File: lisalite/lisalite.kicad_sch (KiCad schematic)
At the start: 4 parts, among them U1 74LS85, U2 74LS393, U3 74LS85, U4 74LS74

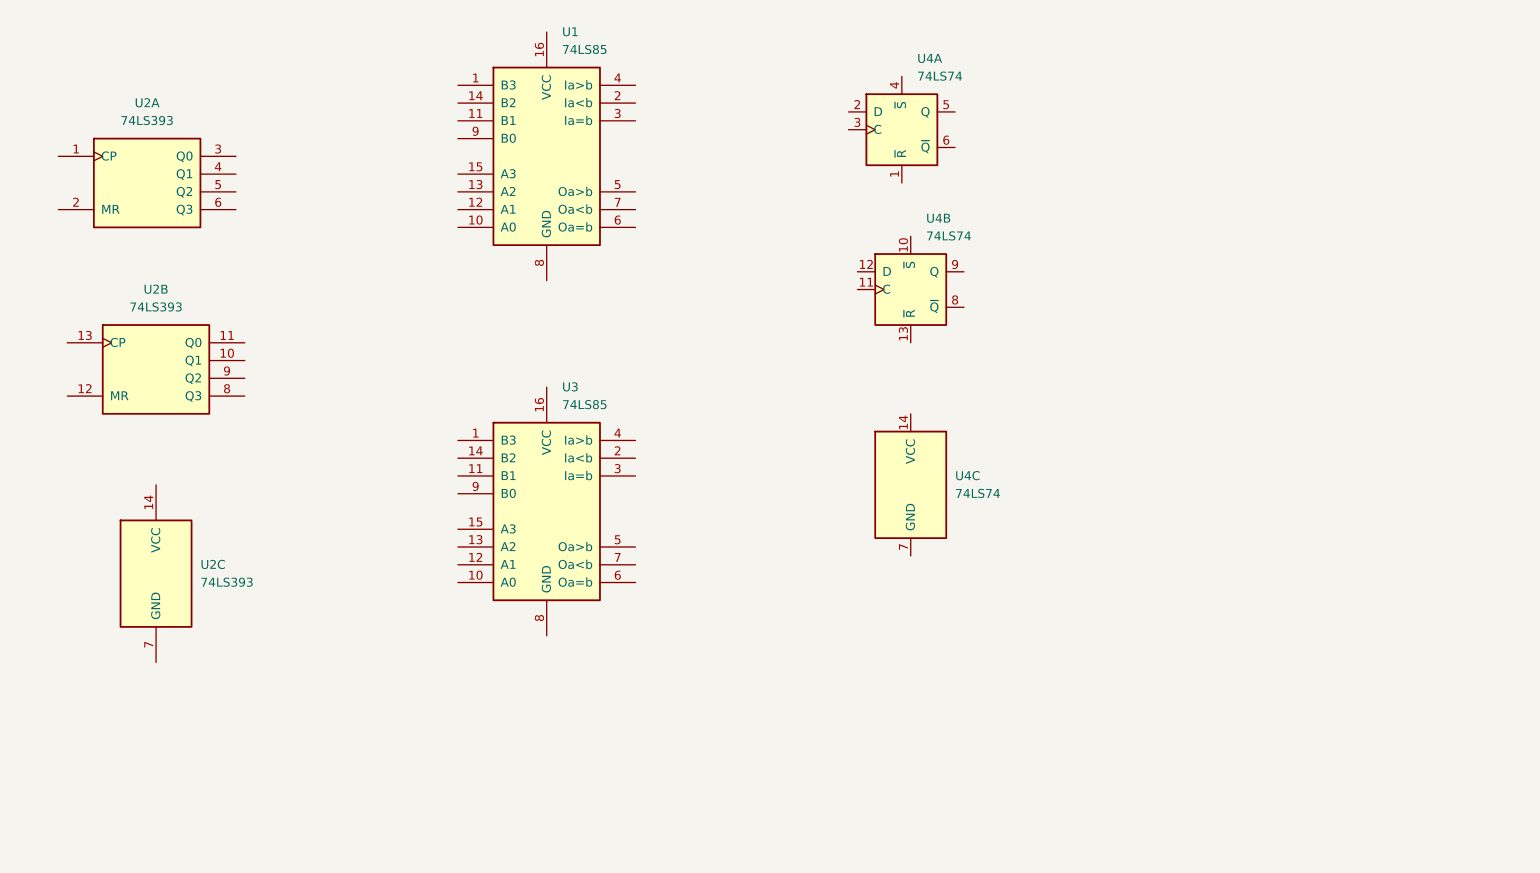
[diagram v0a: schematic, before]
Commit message: schematic updates
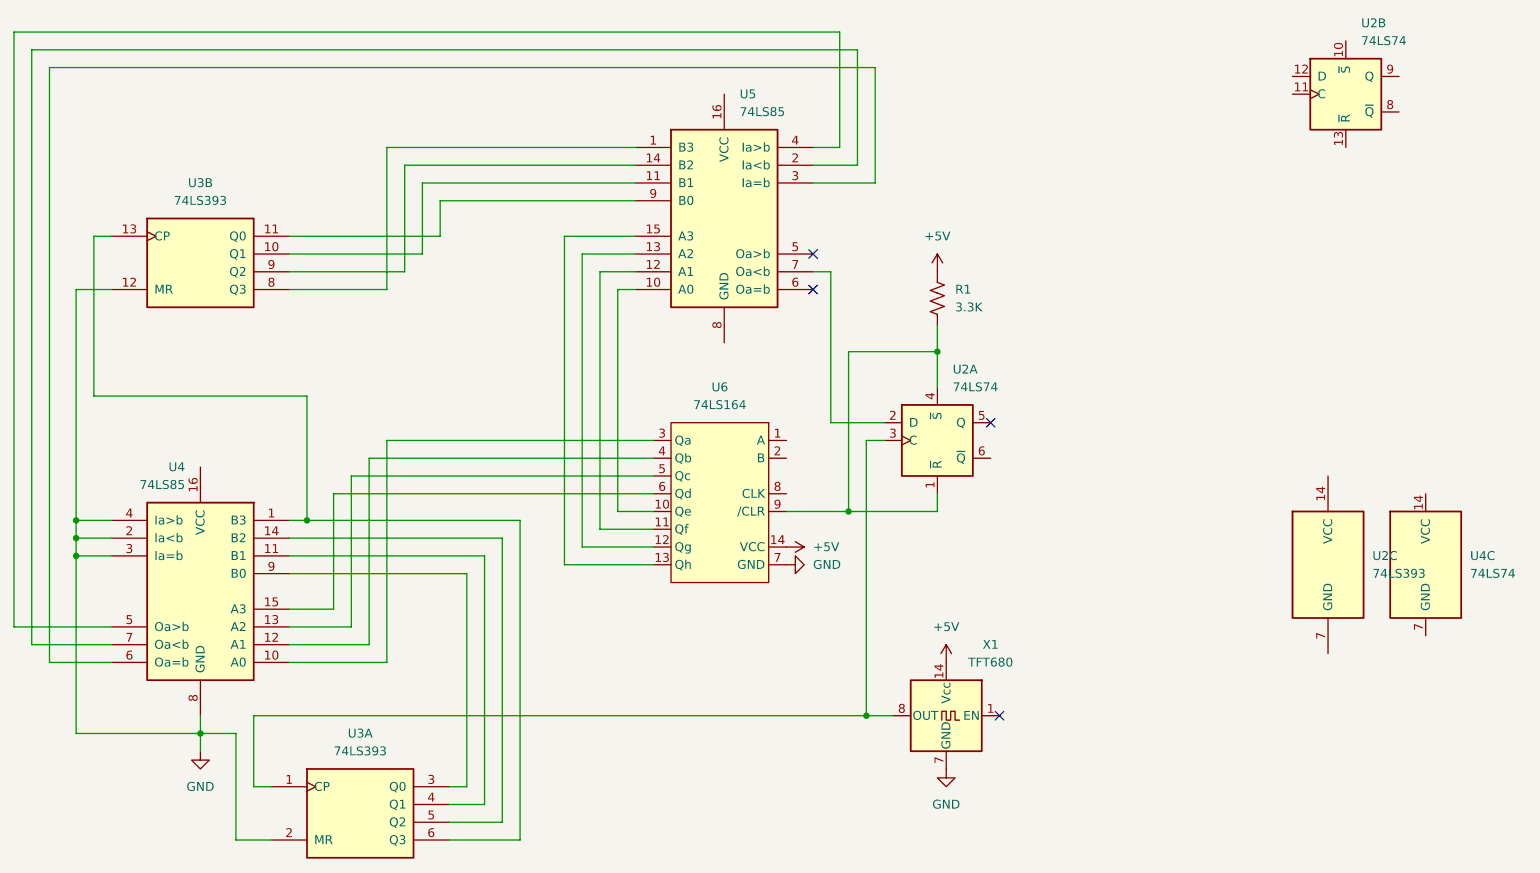
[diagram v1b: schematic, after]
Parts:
- added R1: 3.3K, symbol Device:R_US
- added U6: 74LS164, Package_DIP:DIP-14_W7.62mm, symbol 74xx_Custom:74LS164
- added X1: TFT680, Crystal:Crystal_AT310_D3.0mm_L10.0mm_Horizontal, symbol Oscillator:TFT680
- renumbered U4 to U2, U2 to U3, U3 to U4, U1 to U5
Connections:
- net at U3.1 (CP): now also U2.3 (C), X1.8 (OUT)
- net GND: now reaches U3.2 (MR)
- net GND: now also U3.12 (MR), U4.2 (Ia<b), U4.3 (Ia=b), U4.4 (Ia>b), U4.8 (GND), U6.7 (GND), X1.7 (GND)
- net at U3.3 (Q0): now also U4.9 (B0)
- net at U3.4 (Q1): now also U4.11 (B1)
- net at U3.5 (Q2): now also U4.14 (B2)
- net at U3.6 (Q3): now also U3.13 (CP), U4.1 (B3)
- net at U5.1 (B3): now also U3.8 (Q3)
- net at U5.10 (A0): now also U6.10 (Qe)
- net at U5.11 (B1): now also U3.10 (Q1)
- net at U5.12 (A1): now also U6.11 (Qf)
- net at U5.13 (A2): now also U6.12 (Qg)
- net at U5.14 (B2): now also U3.9 (Q2)
- net at U5.15 (A3): now also U6.13 (Qh)
- net at U5.2 (Ia<b): now also U4.7 (Oa<b)
- net at U5.3 (Ia=b): now also U4.6 (Oa=b)
- net at U5.4 (Ia>b): now also U4.5 (Oa>b)
- net at U5.7 (Oa<b): now also U2.2 (D)
- net at U5.9 (B0): now also U3.11 (Q0)
- net at U4.10 (A0): now also U6.3 (Qa)
- net at U4.12 (A1): now also U6.4 (Qb)
- net at U4.13 (A2): now also U6.5 (Qc)
- net at U4.15 (A3): now also U6.6 (Qd)
- net at U2.1 (~{R}): now also U2.4 (~{S}), R1.2, U6.9 (/CLR)
- new net +5V: R1.1, U6.14 (VCC), X1.14 (Vcc)
- no-connect marks 0 -> 4
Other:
- moved on the sheet: U2A, U2B, U2C, U3A, U3B, U4, U4C, U5
